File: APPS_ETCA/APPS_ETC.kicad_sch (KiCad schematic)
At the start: 18 parts, among them P1 DTM1312PC12PDR008, U3 MCP6004, U6 LM7805_TO220, U8 LM7809_TO220

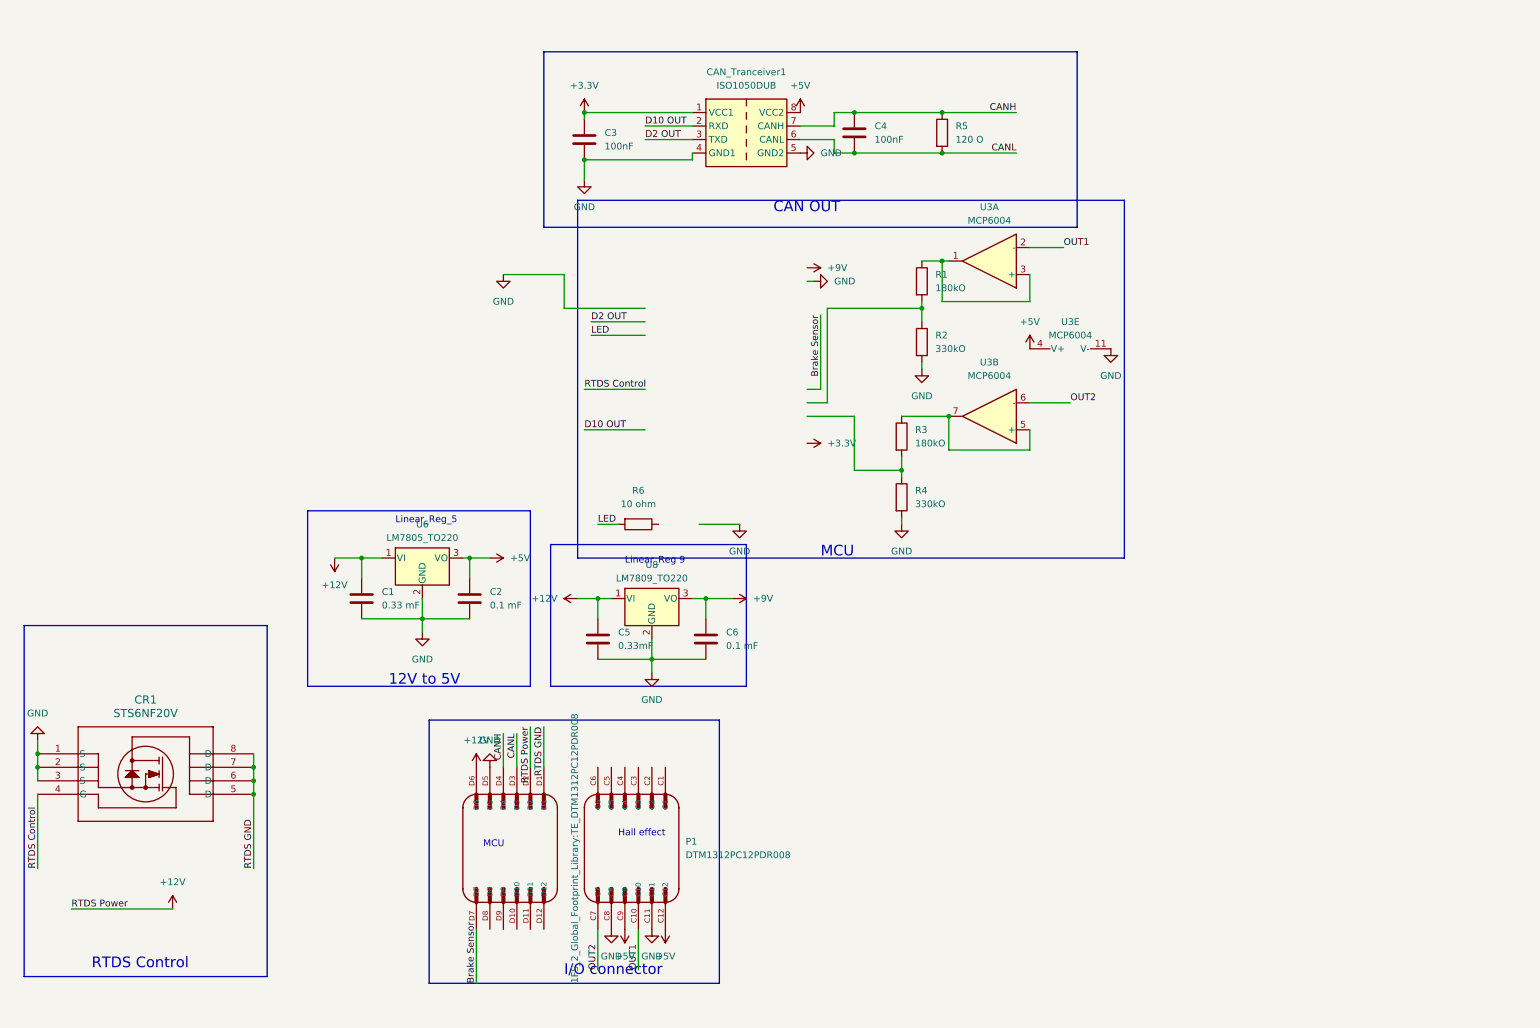
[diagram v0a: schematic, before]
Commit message: LEGGO
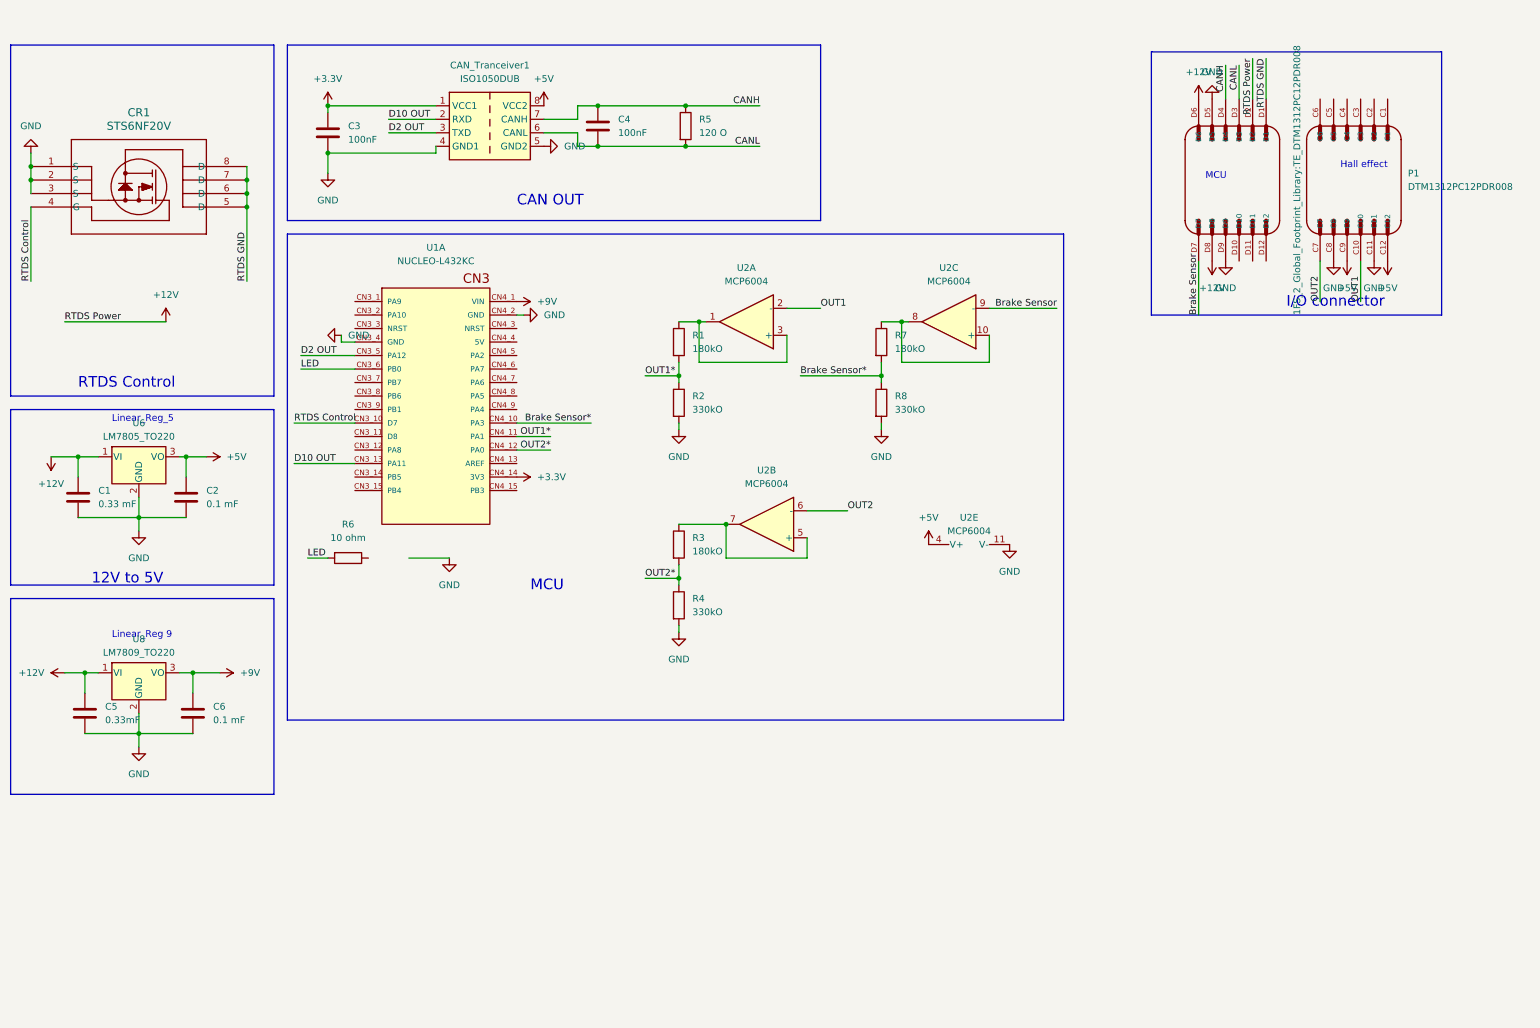
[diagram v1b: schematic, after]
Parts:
- removed U3: MCP6004, FSFootprints:PDIP14_300MC_MCH, symbol Amplifier_Operational:MCP6004
- added R7: 180kO, Resistor_SMD:R_0805_2012Metric_Pad1.20x1.40mm_HandSolder, symbol Device:R
- added R8: 330kO, Resistor_SMD:R_0805_2012Metric_Pad1.20x1.40mm_HandSolder, symbol Device:R
- added U1: NUCLEO-L432KC, 1FS_2_Global_Footprint_Library:MODULE_NUCLEO-L432KC, symbol 1FS_2_Global_Symbol_Library:NUCLEO-L432KC
- added U2: MCP6004, FSFootprints:PDIP14_300MC_MCH, symbol Amplifier_Operational:MCP6004
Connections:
- net +12V: now also P1.D8
- net +3.3V: now also U1.CN4_14 (3V3)
- net +5V: now also U2.4 (V+)
- net +9V: now also U1.CN4_1 (VIN)
- net Brake Sensor: now also U2.9 (-)
- net D10 OUT: now also U1.CN3_13 (PA11)
- net D2 OUT: now also U1.CN3_5 (PA12)
- net GND: now also P1.D9, R8.2, U1.CN3_4 (GND), U1.CN4_2 (GND), U2.11 (V-)
- net LED: now also U1.CN3_6 (PB0)
- net OUT1: now also U2.2 (-)
- net OUT2: now also U2.6 (-)
- net RTDS Control: now also U1.CN3_10 (D7)
- net at R1.1: now also U2.1, U2.3 (+)
- net OUT1*: now reaches R1.2, R2.1
- net OUT1*: now also U1.CN4_11 (PA1)
- net at R3.1: now also U2.5 (+), U2.7
- net OUT2*: now reaches R3.2, R4.1
- net OUT2*: now also U1.CN4_12 (PA0)
- new net: R7.1, U2.10 (+), U2.8
- new net Brake Sensor*: R7.2, R8.1, U1.CN4_10 (PA3)
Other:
- moved on the sheet: C1, C2, C3, C4, C5, C6, CAN_Tranceiver1, CR1, P1, R1, R2, R3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
